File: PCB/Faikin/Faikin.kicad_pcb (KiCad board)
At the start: 2 copper layers, 70 x 70 mm, 31 parts, among them J1 1x5, J2 TC2030-USB-NL-DS, J3 Reset, Q1 BSS138PS, U3 MD8942, U4 ESP32-S3-MINI-1

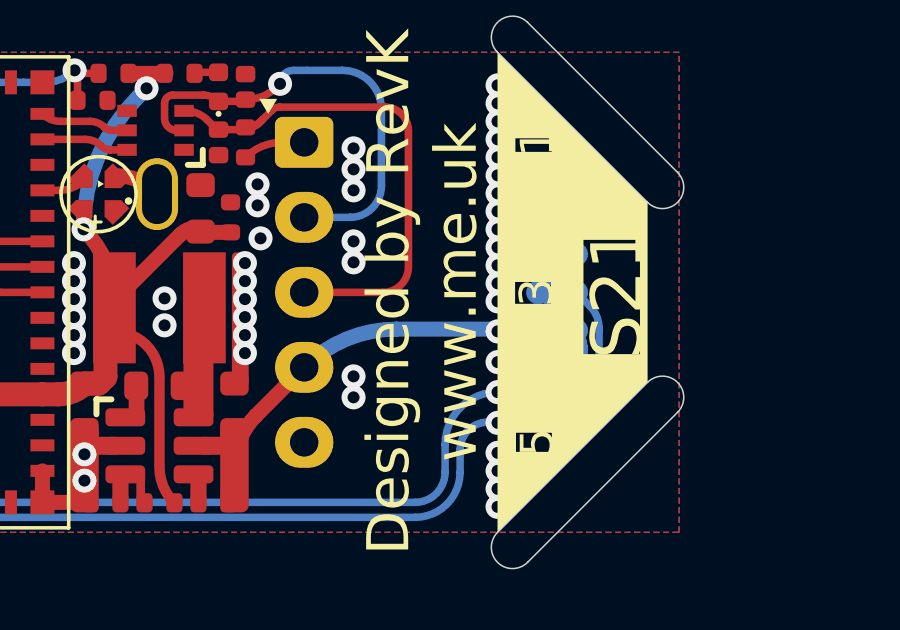
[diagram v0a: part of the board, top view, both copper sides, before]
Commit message: Tidy
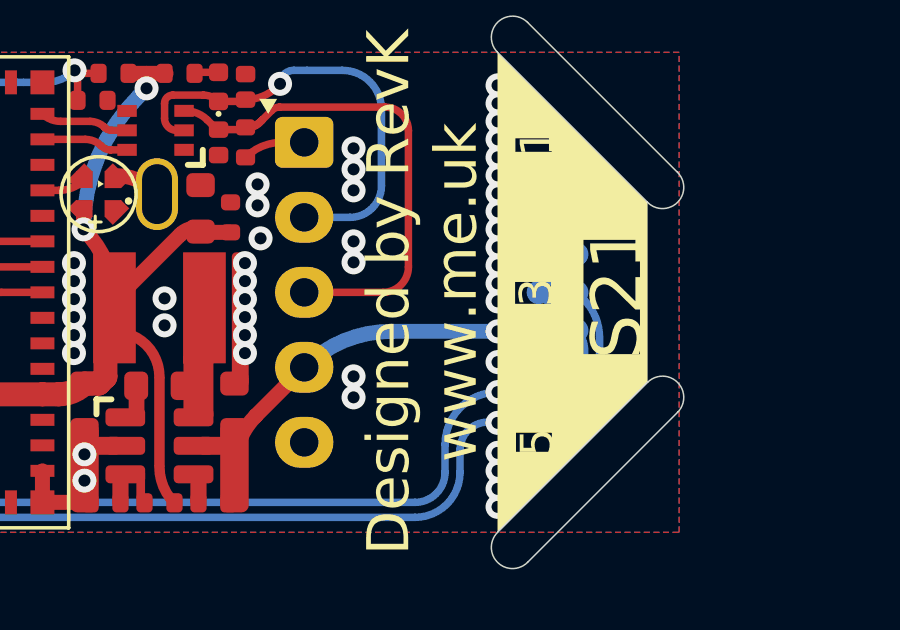
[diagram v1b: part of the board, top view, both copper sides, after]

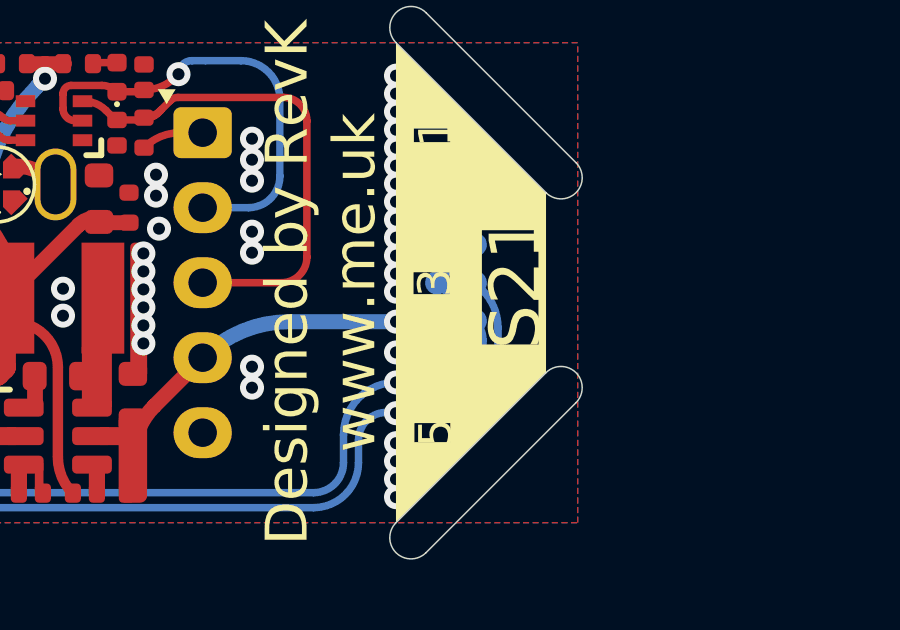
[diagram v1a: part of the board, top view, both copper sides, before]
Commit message: favicon.ico
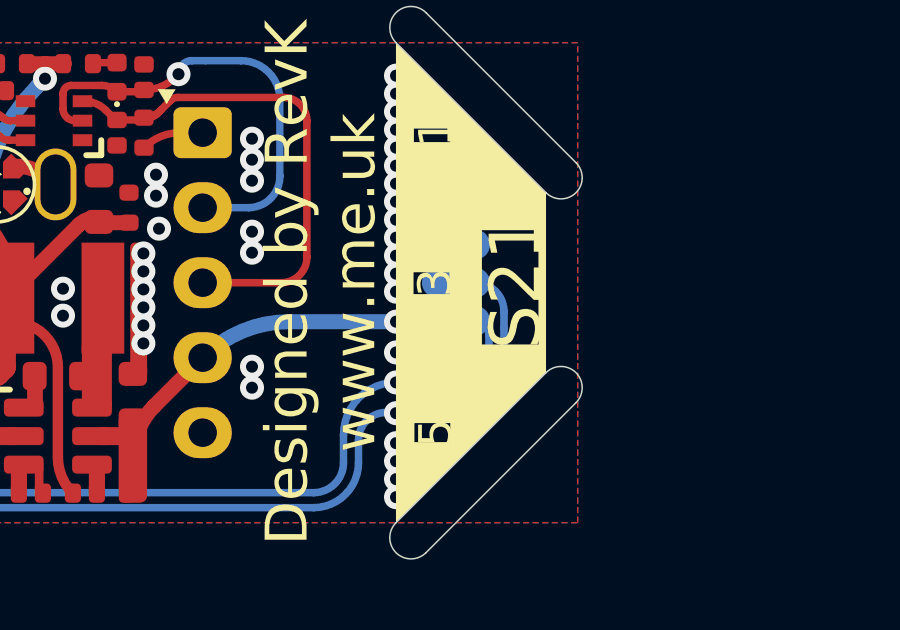
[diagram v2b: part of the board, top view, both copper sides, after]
